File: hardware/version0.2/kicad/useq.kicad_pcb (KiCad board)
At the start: 2 copper layers, 40.6 x 108 mm, 60 parts, among them J1 AudioJack2_SwitchT, J10 Conn_01x03, J11 Conn_01x05, J2 AudioJack2_SwitchT, J3 AudioJack2_SwitchT, J4 AudioJack2_SwitchT, J5 AudioJack2_SwitchT, J6 AudioJack2_SwitchT, J7 AudioJack2_SwitchT, J8 AudioJack2_SwitchT, J9 PJ366ST, Q1 2N3904, Q2 2N3904, SW1 SW_Push, SW2 SW_Push, SW3 SW_SPST, SW4 SW_SPST, U1 Pico, U2 4504

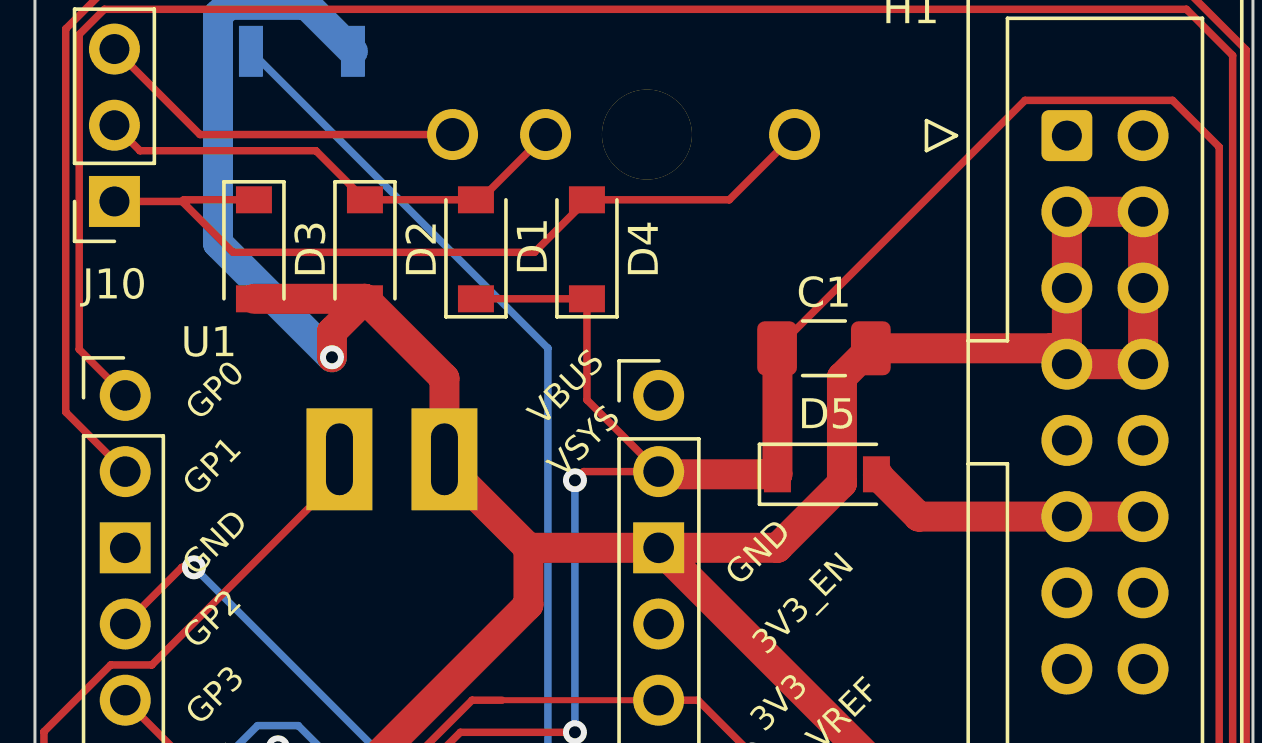
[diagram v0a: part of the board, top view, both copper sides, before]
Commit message: hardware updates
fr4panel, alu panel, jlcpcb production files
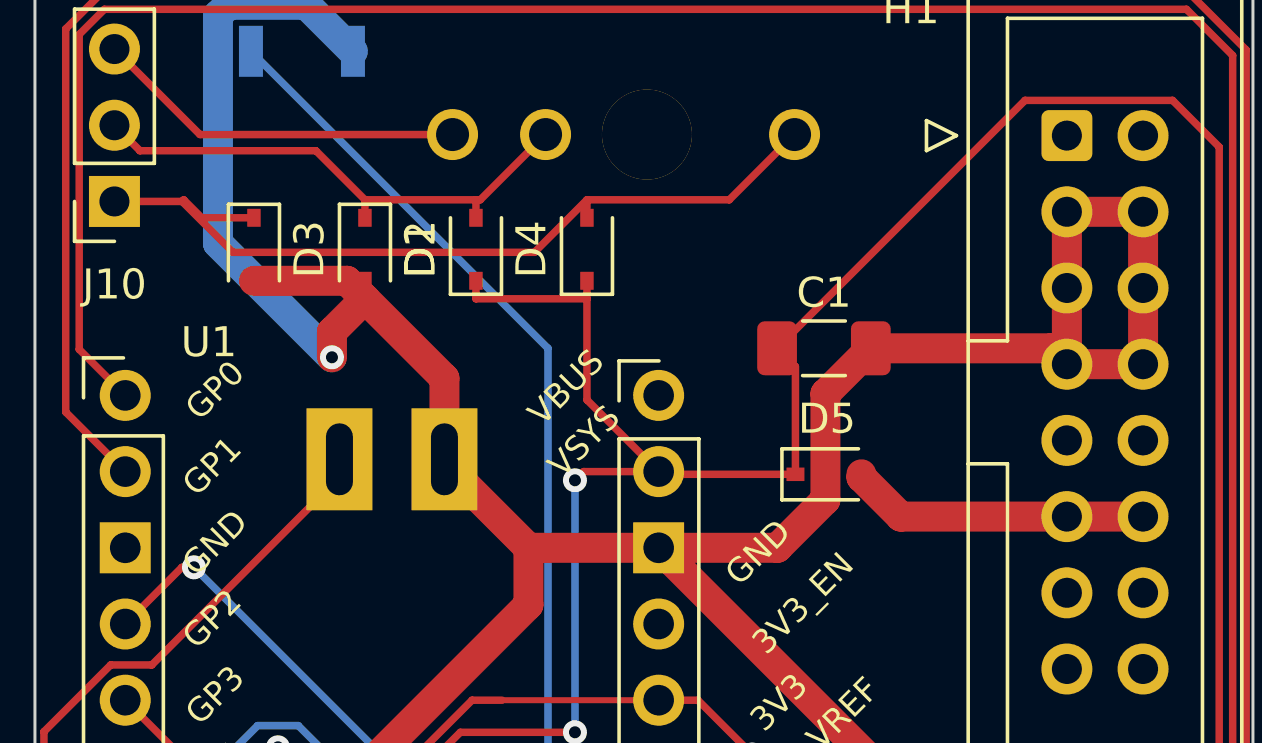
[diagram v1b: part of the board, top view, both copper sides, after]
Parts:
- C3, C4: value 4.7n -> 10n
- C5, C6, C7, C8: value (4.7n) -> (10n)
- D1, D2, D3, D4, D5: footprint Diode_SMD:D_SOD-123 -> Diode_SMD:D_SOD-323
- R10, R11, R12, R13, R14, R7, R8, R9: value 910 -> 1k
- R3, R4: value 2k2 -> 1k
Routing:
- net /5V: track 139.8 -> 142.0 mm
- net Net-(D1-Pad2): track 16.3 -> 17.5 mm
- net Net-(D3-Pad1): track 27.4 -> 28.3 mm
- net Net-(D5-Pad2): track 9.45 -> 10.0 mm
